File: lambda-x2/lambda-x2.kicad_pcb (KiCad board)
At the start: 4 copper layers, 87 x 106 mm, 212 parts, among them J1 FTSH-107-01-F-DV-K, J3 Conn_02x02_Odd_Even, J4 Conn_01x10, P1 33311-24AW-2, Q1 BTS3028, Q2 BTS3028, Q3 BTS3028, Q4 BTS3028, U1 MAX31855KASA, U10 MCP6002T-I/SN, U11 GS8332-SR, U12 MCP6002T-I/SN, U13 MCP6002T-I/SN, U14 MAX31855KASA, U15 MAX31856, U16 MAX31856, U17 MCP6002T-I/SN, U2 STM32F103C6Tx, U3 MCP6002T-I/SN, U4 LM78M05_TO252, U5 XC6206P332MR, U6 REF3033, U7 MCP6002T-I/SN, U8 TJA1051T-3, U9 GS8332-SR

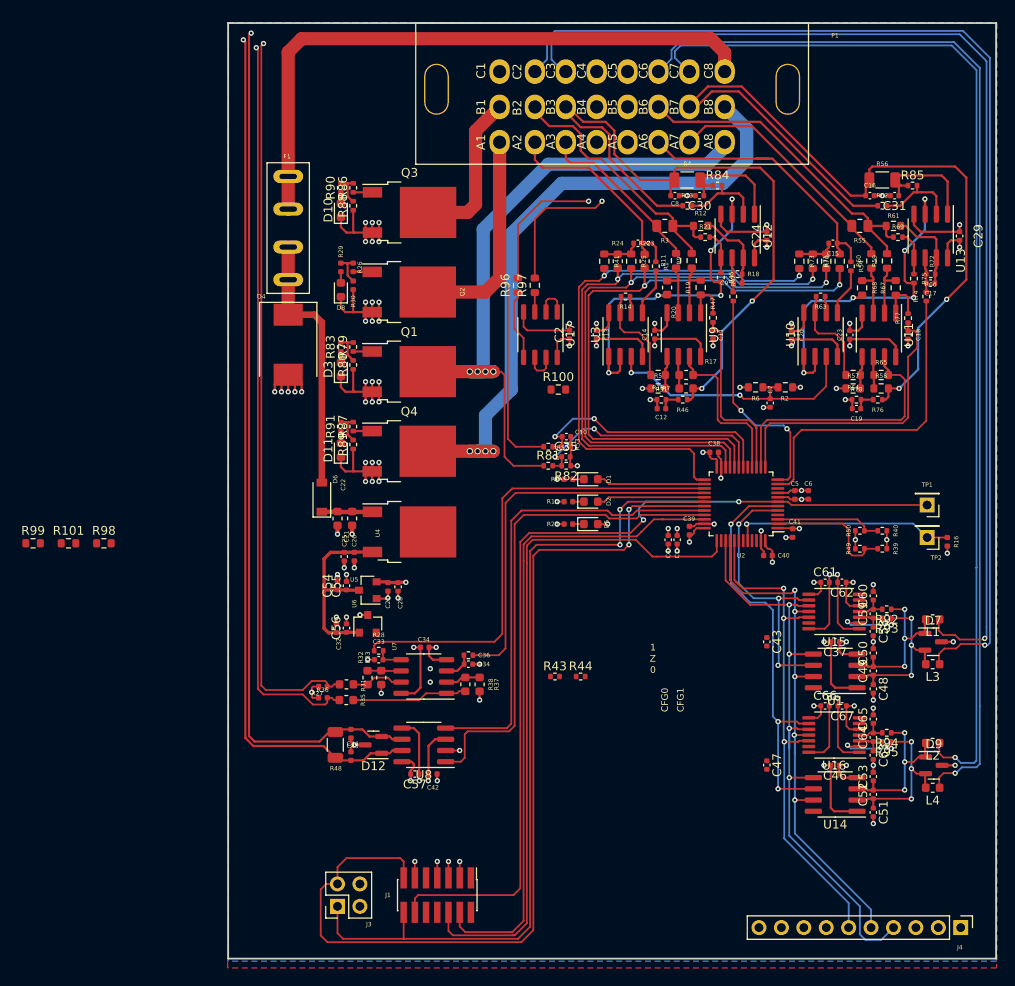
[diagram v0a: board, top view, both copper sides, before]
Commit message: Progress
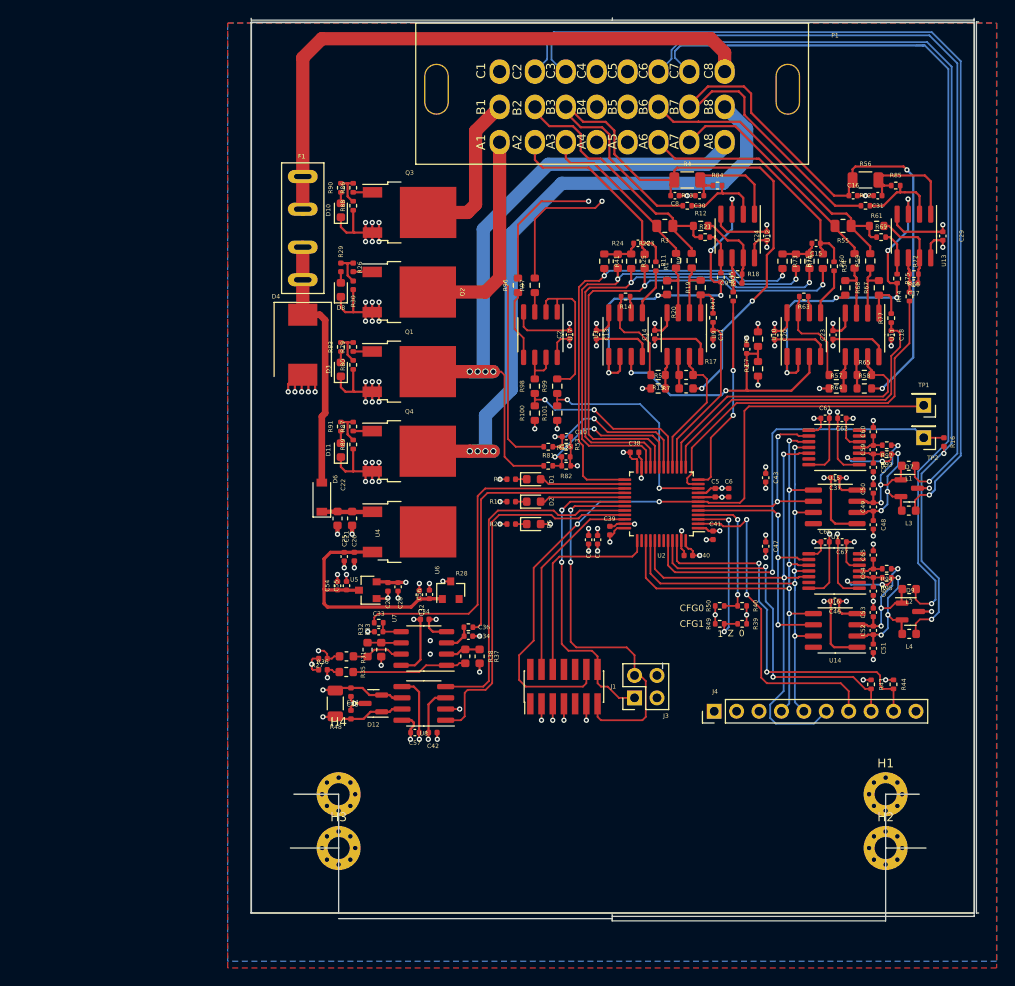
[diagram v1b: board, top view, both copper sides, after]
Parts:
- removed C12, C19: 100n, Capacitor_SMD:C_0402_1005Metric
- removed R46, R76: 100k 1%, Resistor_SMD:R_0402_1005Metric
- removed R51, R78: 10k 1%, Resistor_SMD:R_0402_1005Metric
- added H1: MountingHole_Pad, MountingHole:MountingHole_2.5mm_Pad_Via, F.Cu at (164.5, 119.3)
- added H2: MountingHole_Pad, MountingHole:MountingHole_2.5mm_Pad_Via, F.Cu at (164.5, 125.3)
- added H3: MountingHole_Pad, MountingHole:MountingHole_2.5mm_Pad_Via, F.Cu at (102.5, 125.3)
- added H4: MountingHole_Pad, MountingHole:MountingHole_2.5mm_Pad_Via, F.Cu at (102.5, 119.3)
- moved R99 62.0 mm to (127.3, 73.0), turned to 90 degrees
- moved R101 57.3 mm to (127.3, 76.1), turned to 90 degrees
- moved R98 52.0 mm to (124.7, 73.0), turned to 90 degrees
- moved J3 41.1 mm to (136.0, 108.3)
- moved J4 37.2 mm to (145.0, 109.9), turned to 90 degrees
- moved R43 35.8 mm to (162.8, 106.8), turned to -90 degrees
- moved R44 35.5 mm to (165.4, 106.8), turned to -90 degrees
- moved J1 27.6 mm to (128.0, 107.1), turned to 90 degrees
- moved C47 24.8 mm to (150.9, 91.2)
- moved C43 18.6 mm to (150.9, 83.4)
- moved C46 18.6 mm to (158.7, 97.4)
- moved C48 18.6 mm to (163.1, 88.7)
- moved C49 18.6 mm to (163.1, 86.7)
- moved C50 18.6 mm to (163.1, 84.7)
- moved C51 18.6 mm to (163.1, 102.7)
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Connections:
- U2 pad 2: /config0 -> /SPI1_CS2
- U2 pad 3: /config1 -> /config0
- U2 pad 38: /SPI1_CS2 -> unconnected-(U2-Pad38)
- U2 pad 4: unconnected-(U2-Pad4) -> /config1
- U2 pad 5: /SPI1_CS0 -> /SPI1_CS1
- U2 pad 6: /SPI1_CS1 -> /SPI1_CS0
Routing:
- net /UART_RX: track 110.6 -> 44.2 mm
- net /UART_TX: track 95.6 -> 35.3 mm
- net /SWCLK: track 78.6 -> 23.4 mm
- net /SWDIO: track 74.1 -> 23.2 mm
- net /I2C1_SDA: track 0.00 -> 42.8 mm, vias 0 -> 2
- net /I2C1_SCL: track 0.00 -> 40.5 mm, vias 0 -> 2
- net /SPI1_CS2: track 0.00 -> 37.4 mm, vias 0 -> 2
- net /R_AUX_ADC: track 0.00 -> 25.9 mm, vias 0 -> 2
- net /Boot0: track 25.3 -> 50.7 mm
- net /L_EGT+: track 127.7 -> 104.0 mm
- net /L_EGT-: track 129.9 -> 107.2 mm
- net /nRESET: track 102.9 -> 80.8 mm
- net /L_AUX_ADC: track 0.00 -> 21.8 mm, vias 0 -> 2
- net /R_EGT-: track 124.9 -> 105.6 mm, vias 1 -> 2
- net /SPI1_CS1: track 47.0 -> 29.3 mm
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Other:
- board size 87 x 106 mm -> 82.4 x 102.3 mm

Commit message: Progress
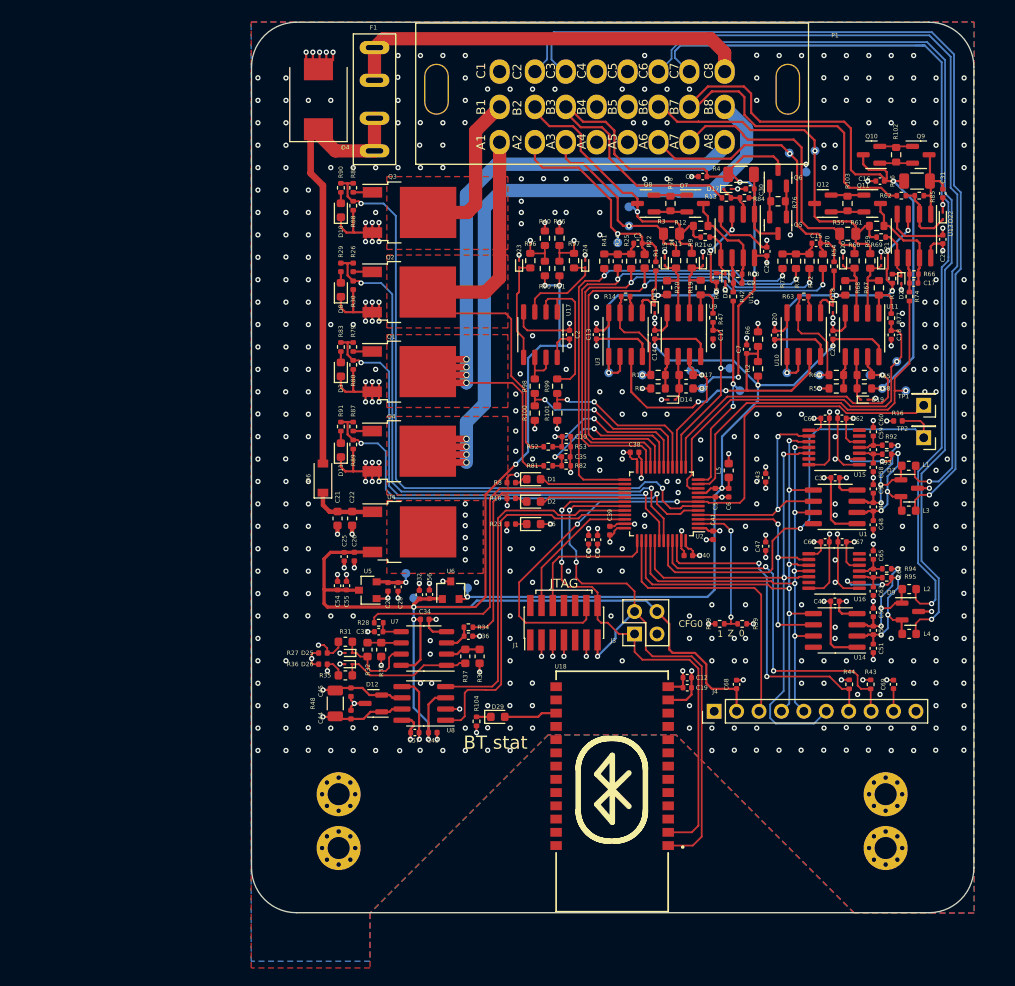
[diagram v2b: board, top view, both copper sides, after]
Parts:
- added C12: 1u, Capacitor_SMD:C_0402_1005Metric, F.Cu at (142.0, 106.0)
- added C19: 100n, Capacitor_SMD:C_0402_1005Metric, F.Cu at (142.0, 107.2)
- added C68: 100n, Capacitor_SMD:C_0402_1005Metric, F.Cu at (147.6, 106.8)
- added C69: 100n, Capacitor_SMD:C_0402_1005Metric, F.Cu at (165.4, 106.8)
- added D13: DF2B7AFS,L3M, Diode_SMD:D_SOD-923, F.Cu at (138.3, 64.3)
- added D14: DF2B7AFS,L3M, Diode_SMD:D_SOD-923, F.Cu at (140.2, 74.5)
- added D15: DF2B7AFS,L3M, Diode_SMD:D_SOD-923, F.Cu at (139.4, 58.9)
- added D16: DF2B7AFS,L3M, Diode_SMD:D_SOD-923, F.Cu at (143.8, 58.9)
- added D17: DF2B7AFS,L3M, Diode_SMD:D_SOD-923, F.Cu at (146.6, 50.7)
- added D18: DF2B7AFS,L3M, Diode_SMD:D_SOD-923, F.Cu at (158.5, 64.3)
- added D19: DF2B7AFS,L3M, Diode_SMD:D_SOD-923, F.Cu at (162.1, 74.5)
- added D20: DF2B7AFS,L3M, Diode_SMD:D_SOD-923, F.Cu at (159.6, 58.9)
- added D21: DF2B7AFS,L3M, Diode_SMD:D_SOD-923, F.Cu at (164.0, 58.9)
- added D22: DF2B7AFS,L3M, Diode_SMD:D_SOD-923, F.Cu at (170.9, 53.7)
- added D23: DF2B7AFS,L3M, Diode_SMD:D_SOD-923, F.Cu at (122.9, 59.2)
- added D24: DF2B7AFS,L3M, Diode_SMD:D_SOD-923, F.Cu at (130.4, 59.2)
- added D25: DF2B7AFS,L3M, Diode_SMD:D_SOD-923, F.Cu at (103.6, 103.3)
- added D26: DF2B7AFS,L3M, Diode_SMD:D_SOD-923, F.Cu at (103.6, 104.5)
- added D27: DF2B7AFS,L3M, Diode_SMD:D_SOD-923, F.Cu at (146.3, 60.7)
- added D28: DF2B7AFS,L3M, Diode_SMD:D_SOD-923, F.Cu at (166.2, 61.0)
- added D29: GREEN, LED_SMD:LED_0603_1608Metric, F.Cu at (120.5, 110.5)
- added L5: 470R@100MHz, Inductor_SMD:L_0603_1608Metric, F.Cu at (146.7, 82.6)
- added Q10: BSS169H6327, Package_TO_SOT_SMD:SOT-23, F.Cu at (162.9, 46.8)
- added Q11: BSS169H6327, Package_TO_SOT_SMD:SOT-23, F.Cu at (162.9, 52.3)
- added Q12: BSS169H6327, Package_TO_SOT_SMD:SOT-23, F.Cu at (157.4, 52.3)
- added Q5: BSS169H6327, Package_TO_SOT_SMD:SOT-23, F.Cu at (152.3, 54.8)
- added Q6: BSS169H6327, Package_TO_SOT_SMD:SOT-23, F.Cu at (152.3, 49.4)
- added Q7: BSS169H6327, Package_TO_SOT_SMD:SOT-23, F.Cu at (142.9, 52.3)
- added Q8: BSS169H6327, Package_TO_SOT_SMD:SOT-23, F.Cu at (137.3, 52.3)
- added Q9: BSS169H6327, Package_TO_SOT_SMD:SOT-23, F.Cu at (168.5, 46.8)
- added R102: 75R, Resistor_SMD:R_0603_1608Metric, F.Cu at (165.7, 46.8)
- added R103: 75R, Resistor_SMD:R_0603_1608Metric, F.Cu at (160.1, 52.3)
- added R104: 1k, Resistor_SMD:R_0402_1005Metric, F.Cu at (118.1, 111.0)
- added R46: 1K, Resistor_SMD:R_0603_1608Metric, F.Cu at (127.5, 56.3)
- added R51: 1K, Resistor_SMD:R_0603_1608Metric, F.Cu at (127.5, 59.7)
- added R76: 75R, Resistor_SMD:R_0603_1608Metric, F.Cu at (152.3, 52.1)
- added R78: 75R, Resistor_SMD:R_0603_1608Metric, F.Cu at (140.1, 52.3)
- added TP10: Ip, TestPoint:TestPoint_Pad_D1.0mm, B.Cu at (135.4, 54.9)
- added TP11: Rtrim, TestPoint:TestPoint_Pad_D1.0mm, B.Cu at (135.4, 52.7)
- added TP12: Vm, TestPoint:TestPoint_Pad_D1.0mm, B.Cu at (143.6, 73.3)
- added TP13: Un, TestPoint:TestPoint_Pad_D1.0mm, B.Cu at (134.1, 56.8)
- added TP14: Un, TestPoint:TestPoint_Pad_D1.0mm, B.Cu at (133.1, 71.5)
- added TP15: Ip_DAC, TestPoint:TestPoint_Pad_D1.0mm, B.Cu at (148.0, 73.5)
- added TP16: Ip_Sense, TestPoint:TestPoint_Pad_D1.0mm, B.Cu at (146.8, 71.0)
- added TP17: Ip, TestPoint:TestPoint_Pad_D1.0mm, B.Cu at (155.4, 48.8)
- added TP18: Rtrim, TestPoint:TestPoint_Pad_D1.0mm, B.Cu at (156.5, 46.4)
- added TP19: Vm, TestPoint:TestPoint_Pad_D1.0mm, B.Cu at (164.1, 73.3)
- added TP20: Un, TestPoint:TestPoint_Pad_D1.0mm, B.Cu at (153.5, 46.6)
- added TP21: Un, TestPoint:TestPoint_Pad_D1.0mm, B.Cu at (153.3, 71.5)
- added TP22: Ip_DAC, TestPoint:TestPoint_Pad_D1.0mm, B.Cu at (166.8, 73.5)
- added TP23: Ip_Sense, TestPoint:TestPoint_Pad_D1.0mm, B.Cu at (165.7, 70.2)
- added TP24: GND, TestPoint:TestPoint_Pad_D1.0mm, B.Cu at (114.3, 90.8)
- added TP3: Un_Sense, TestPoint:TestPoint_Pad_D1.0mm, B.Cu at (136.9, 71.8)
- added TP4: Un_Sense, TestPoint:TestPoint_Pad_D1.0mm, B.Cu at (157.0, 71.8)
- added TP5: 3xUn, TestPoint:TestPoint_Pad_D1.0mm, B.Cu at (142.4, 71.2)
- added TP6: 3xUn, TestPoint:TestPoint_Pad_D1.0mm, B.Cu at (162.7, 71.8)
- added TP7: 5V, TestPoint:TestPoint_Pad_D1.0mm, B.Cu at (111.0, 97.0)
- added TP8: 3V3, TestPoint:TestPoint_Pad_D1.0mm, B.Cu at (110.1, 94.2)
- added TP9: Vdda, TestPoint:TestPoint_Pad_D1.0mm, B.Cu at (117.1, 95.9)
- added U18: JDY-33, local:JDY-33, F.Cu at (133.5, 118.7)
- R40: value 0R -> 1K; footprint Resistor_SMD:R_0402_1005Metric -> Resistor_SMD:R_0603_1608Metric
- R50: value 10k -> 1K; footprint Resistor_SMD:R_0402_1005Metric -> Resistor_SMD:R_0603_1608Metric
- moved R40 47.3 mm to (125.9, 56.3), turned to 90 degrees
- moved R50 43.1 mm to (125.9, 59.7), turned to 90 degrees
- moved D4 27.9 mm to (100.2, 40.5), turned to 90 degrees
- moved F1 16.7 mm to (106.6, 40.5)
- moved C31 7.37 mm to (170.9, 51.2), turned to -90 degrees
- moved J1 7.24 mm to (128.0, 99.8)
- moved J3 7.24 mm to (136.0, 101.1)
- moved R4 6.13 mm to (148.1, 49.0)
- moved R56 5.84 mm to (168.0, 49.8)
- moved C30 5.77 mm to (149.1, 50.7)
- moved R16 5.73 mm to (165.9, 77.0), turned to 0 degrees
- moved R97 5.25 mm to (129.2, 58.8)
- moved R44 5.02 mm to (160.3, 106.8)
- moved R13 4.53 mm to (146.4, 51.7)
- moved R62 4.22 mm to (166.2, 51.4)
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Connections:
- J4 pad 3: unconnected-(J4-Pad3) -> /SPI1_CS2
- J4 pad 7: /SPI1_CS2 -> /I2C1_SDA
- J4 pad 9: /I2C1_SDA -> +3V3
- R40 pad 1: /config1 -> /L_AUX
- R50 pad 1: /config1 -> +5V
- R50 pad 2: +3V3 -> /L_AUX
- U2 pad 10: /R_AUX_ADC -> /R_Ip_sense
- U2 pad 13: /R_Ip_sense -> /R_Un_3x_sense
- U2 pad 14: /R_Un_3x_sense -> /L_Ip_sense
- U2 pad 15: /L_Ip_sense -> /L_Un_3x_sense
- U2 pad 16: /L_Un_3x_sense -> /R_AUX_ADC
- U2 pad 2: /SPI1_CS2 -> /config0
- U2 pad 3: /config0 -> /SPI1_CS1
- U2 pad 38: unconnected-(U2-Pad38) -> /SPI1_CS2
- U2 pad 4: /config1 -> /SPI1_CS0
- U2 pad 42: /L_heater_pwm -> /R_heater_pwm
- U2 pad 43: /R_heater_pwm -> /L_heater_pwm
- U2 pad 5: /SPI1_CS1 -> /R_OUT_en
- U2 pad 6: /SPI1_CS0 -> /L_OUT_en
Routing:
- net +5V: track 46.9 -> 164.0 mm, vias 3 -> 7
- net VDDA: track 19.9 -> 100.7 mm, vias 4 -> 5
- net /L_OUT_en: track 3.74 -> 76.2 mm, vias 0 -> 2
- net /L_heater_pwm: track 3.74 -> 66.6 mm, vias 0 -> 2
- net /R_heater_pwm: track 3.69 -> 56.8 mm, vias 0 -> 2
- net /R_OUT_en: track 3.69 -> 50.0 mm, vias 0 -> 2
- net /UART_TX: track 35.3 -> 59.6 mm
- net /UART_RX: track 44.2 -> 68.1 mm, vias 2 -> 3
- net 12V_RAW: track 68.7 -> 46.6 mm
- net 12V_PROT: track 29.0 -> 50.2 mm
- net GND: track 253.0 -> 274.1 mm, vias 100 -> 472
- net /R_LSU_Heater-: track 75.1 -> 92.1 mm
- net /config1: track 16.0 -> 0.00 mm, vias 2 -> 0
- net /R_OD: track 73.1 -> 87.5 mm
- net /R_LSU_Vm: track 90.5 -> 100.1 mm
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- added copper zone on F.Cu, net /L_LSU_Heater-
- added copper zone on F.Cu, net /L_OD
- added copper zone on F.Cu, net /R_LSU_Heater-
- added copper zone on F.Cu, net /R_OD
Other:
- board size 82.4 x 102.3 mm -> 81.8 x 100.9 mm
- board text added: "+5V"
- board text added: "BT stat"
- board text added: "CS"
- board text added: "JTAG"
- board text added: "MISO"
- board text added: "MOSI"
- board text added: "RX"
- board text added: "RusEFI Lambda X2 Rev 0 https://github.com/dron0gus/"
- board text added: "SCK"
- board text added: "SCL"
- board text added: "SDA"
- board text added: "TX"
- board text removed: "+12V"
- board text removed: "CAN_H"
- board text removed: "CAN_L"
- board text removed: "CFG1"
- board text removed: "F103 Wideband rev 2 http://www.github.com/s/wb"
- board text removed: "GND +5V"
- board text removed: "Heater+ grey"
- board text removed: "Heater- white"
- board text removed: "Ip red"
- board text removed: "PA15"
- board text removed: "PB3"
- board text removed: "PB4"
- board text removed: "PB5"
- board text removed: "PB7"
- board text removed: "PB8"
- board text removed: "PB9"
- board text removed: "Rtrim green"
- board text removed: "TX RX"
- board text removed: "Un black"
- board text removed: "Vm yellow"
- board text removed: "Vout1"
- board text removed: "Vout2"
